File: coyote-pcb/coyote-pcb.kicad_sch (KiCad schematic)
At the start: 7 parts

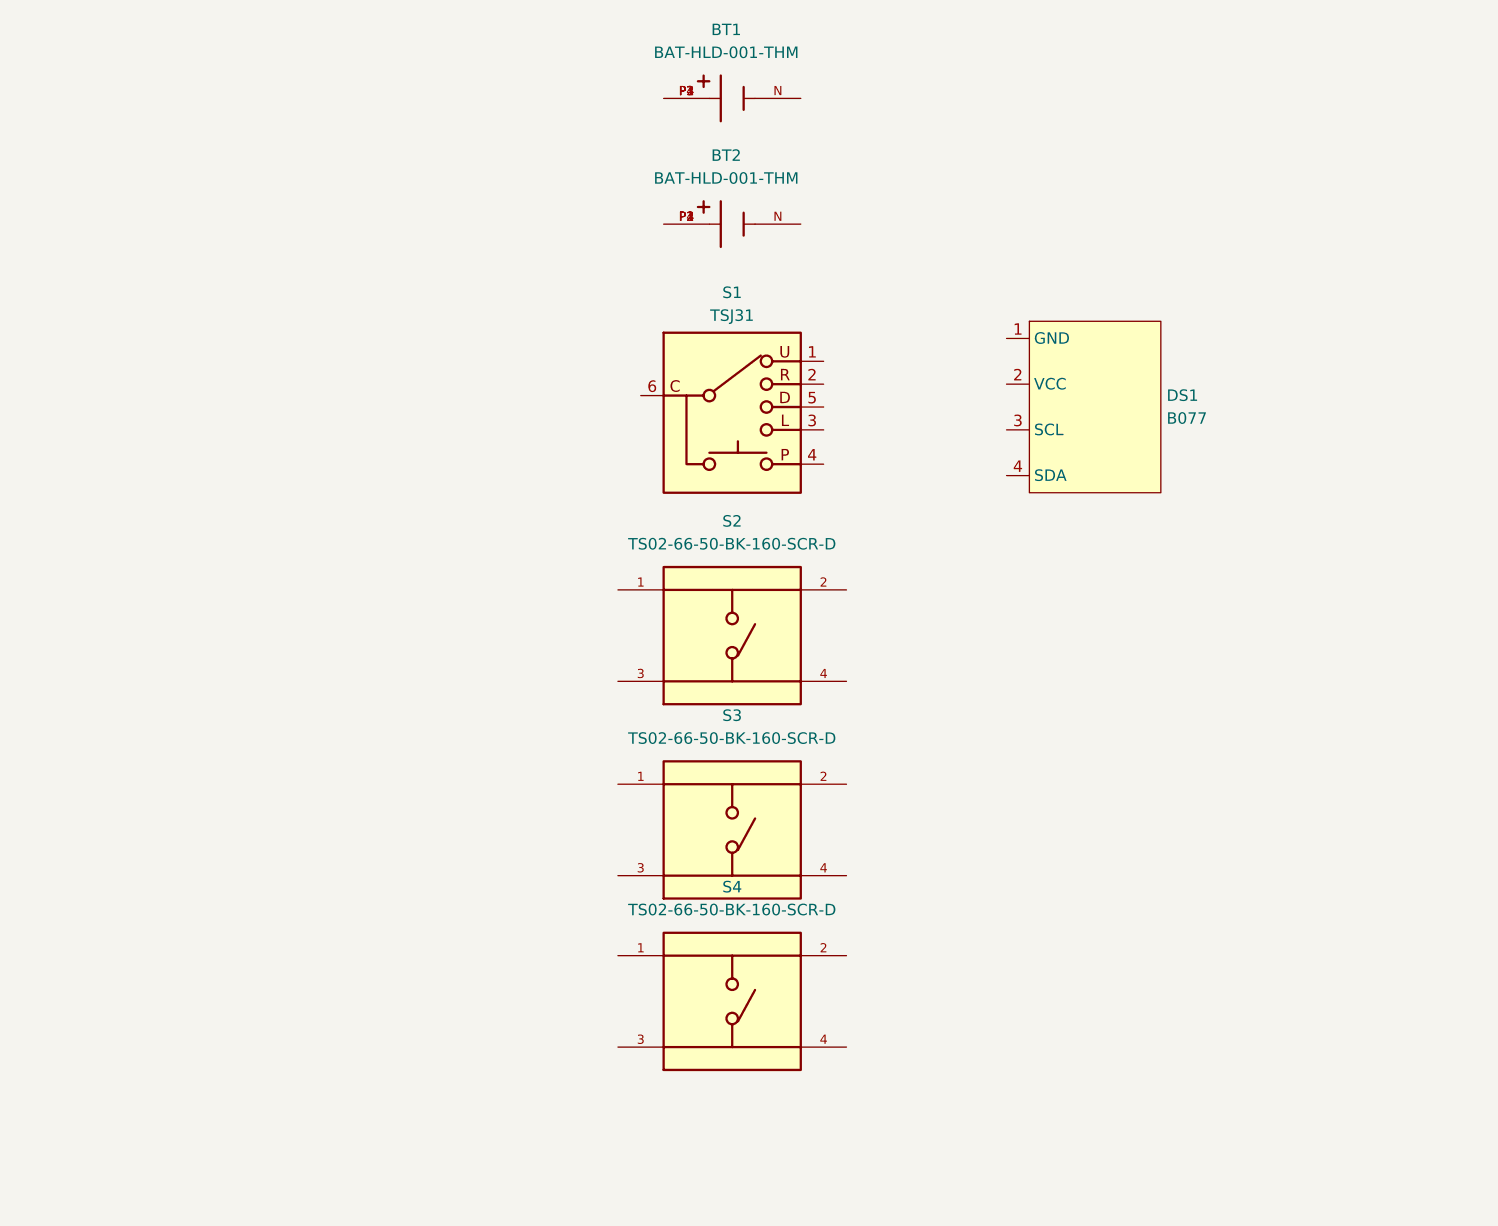
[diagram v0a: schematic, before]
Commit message: First full pass at design. Update gitignore.
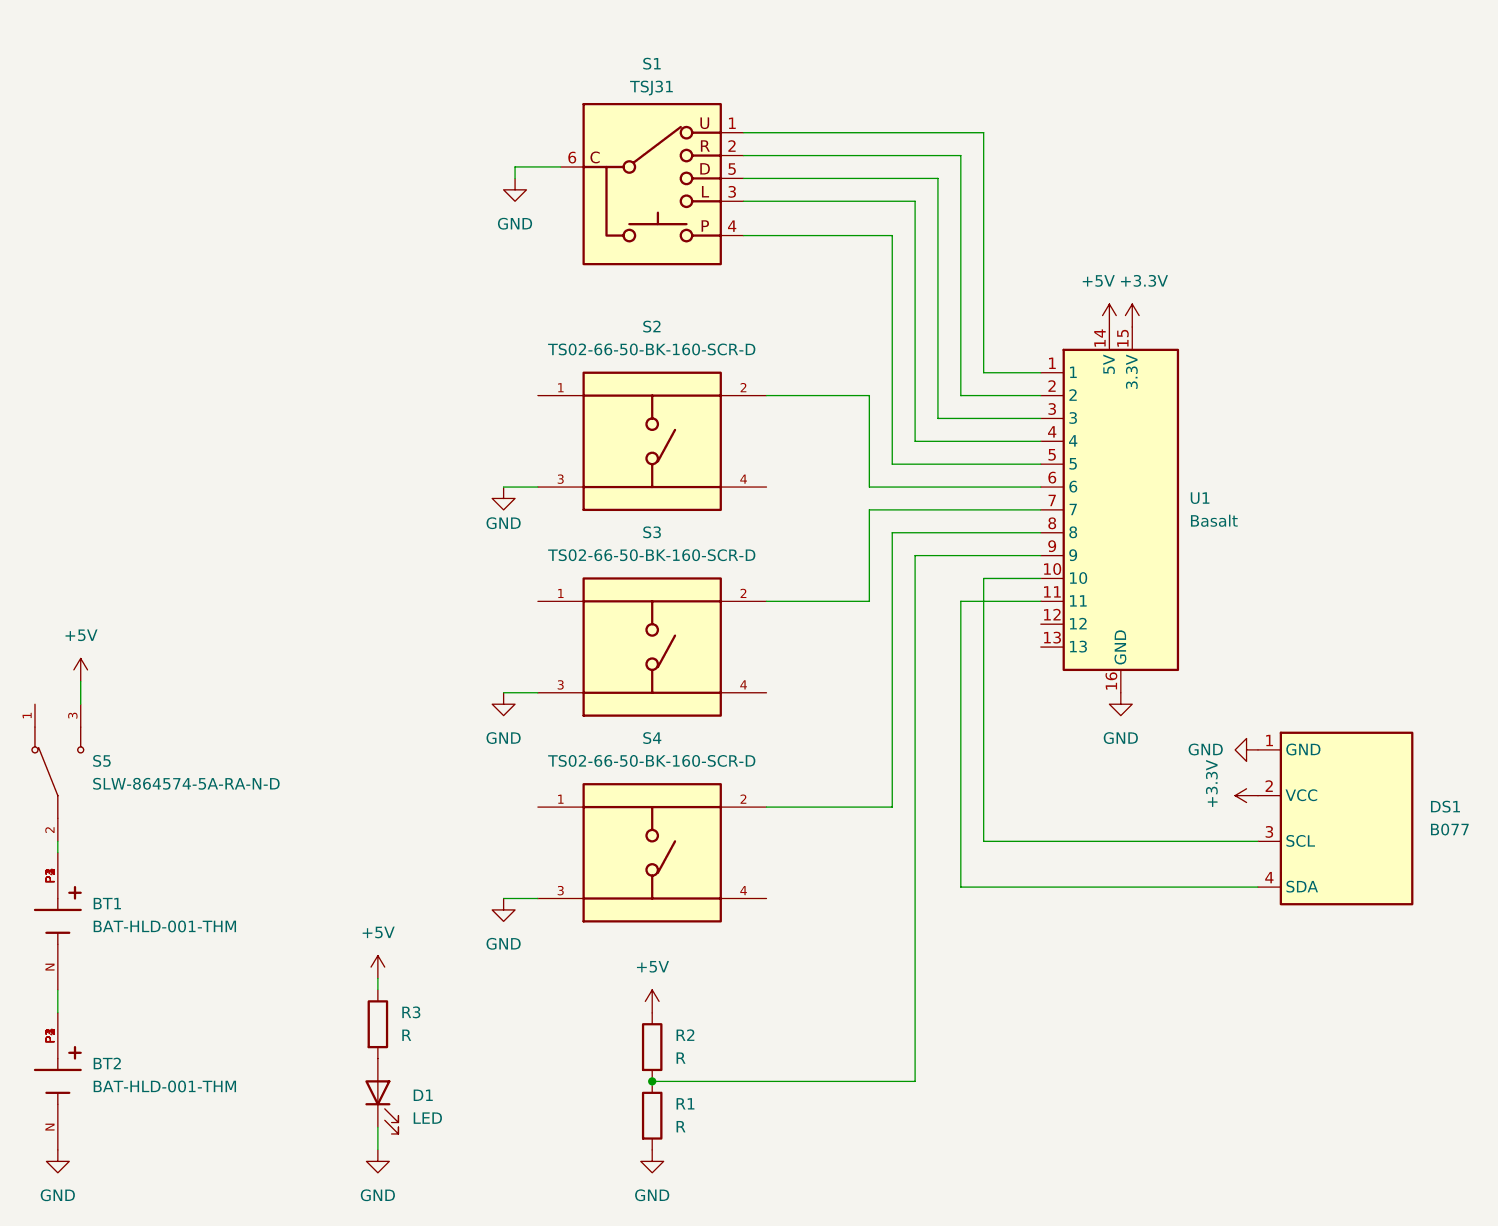
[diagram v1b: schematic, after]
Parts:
- added D1: LED, LED_THT:LED_D3.0mm, symbol Device:LED
- added R1, R2, R3: R, Resistor_THT:R_Axial_DIN0309_L9.0mm_D3.2mm_P12.70mm_Horizontal, symbol Device:R
- added S5: SLW-864574-5A-RA-N-D, my-kicad-parts:SW_SLW-864574-5A-RA-N-D, symbol my-kicad-parts:SLW-864574-5A-RA-N-D
- added U1: Basalt, my-kicad-parts:MESA_Basalt, symbol my-kicad-parts:MESA_Basalt
- BT1, BT2: footprint BAT-HLD-001-THM:BAT_BAT-HLD-001-THM -> my-kicad-parts:BAT_BAT-HLD-001-THM
- DS1: footprint (none) -> my-kicad-parts:B077
- S1: footprint (none) -> my-kicad-parts:TSJ31
- S2, S3, S4: footprint TS02-66-50-BK-160-SCR-D:SW_TS02-66-50-BK-160-SCR-D -> my-kicad-parts:SW_TS02-66-50-BK-160-SCR-D
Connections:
- net GND: now reaches DS1.1 (GND)
- net GND: now also BT2.N, S1.6 (COMMON), S2.3, S3.3, S4.3, D1.1 (K), R1.2, U1.16 (GND)
- net +3.3V: now reaches DS1.2 (VCC)
- net +3.3V: now also U1.15 (3.3V)
- net at DS1.3 (SCL): now also U1.10
- net at DS1.4 (SDA): now also U1.11
- net at S1.1 (UP): now also U1.1
- net at S1.2 (RIGHT): now also U1.2
- net at S1.3 (LEFT): now also U1.4
- net at S1.4 (PRESS): now also U1.5
- net at S1.5 (DOWN): now also U1.3
- net at BT2.P1, BT2.P2, BT2.P3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: now also BT1.N
- net at S4.2: now also U1.8
- net at BT1.P1, BT1.P2, BT1.P3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: now also S5.2
- net at S3.2: now also U1.7
- net at S2.2: now also U1.6
- new net: D1.2 (A), R3.2
- new net: R1.1, R2.2, U1.9
- new net +5V: R2.1, R3.1, S5.3, U1.14 (5V)
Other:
- moved on the sheet: BT1, BT2, S1, S2, S3, S4
